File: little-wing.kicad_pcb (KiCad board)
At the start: 2 copper layers, 116.8 x 96 mm, 72 parts, among them IC1 AP7335-WG-7, J1 nice!view, J2 Battery, J3 trackball, J4 trackball, SW1 Power, SW2 Reset, U1 nice!nano v2, U2 PMW3610

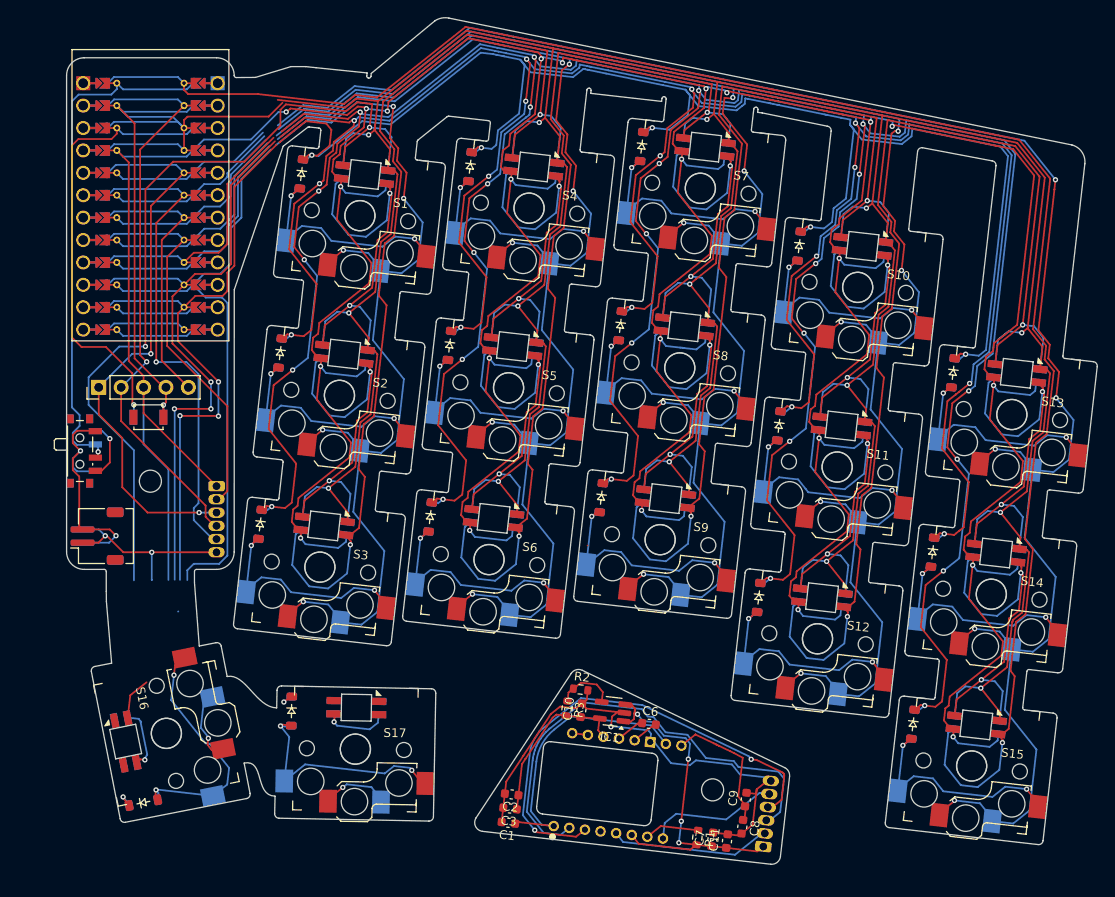
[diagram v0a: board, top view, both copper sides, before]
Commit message: Finalizing the wiring
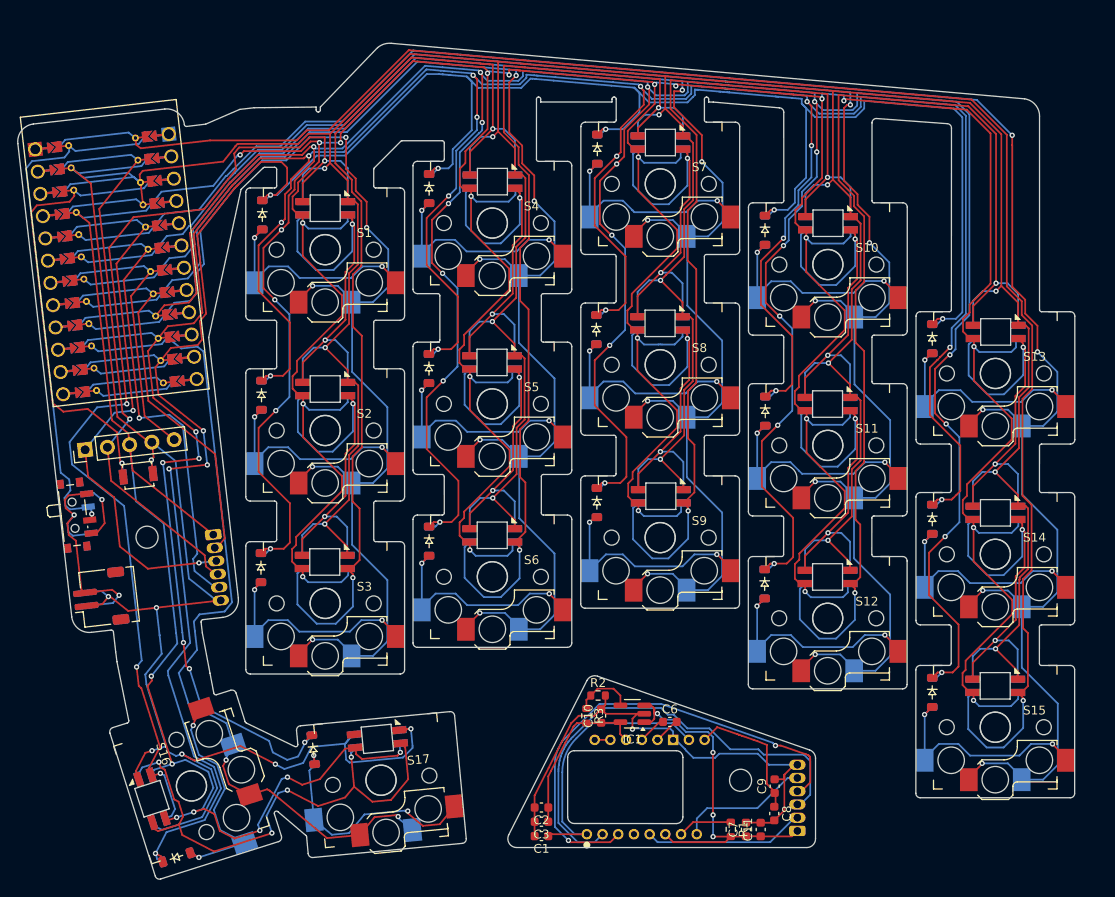
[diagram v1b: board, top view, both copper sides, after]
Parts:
- moved U1 7.63 mm to (102.3, 74.2), turned to -83.5 degrees
- moved SW1 7.28 mm to (97.8, 102.6), turned to -83.5 degrees
- moved D16 7.25 mm to (109.1, 141.4), turned to 18 degrees
- moved J1 7.25 mm to (98.8, 95.2), turned to 96.5 degrees
- moved D19 7.13 mm to (106.4, 134.8), turned to 108 degrees
- moved J2 7.00 mm to (100.5, 112.0), turned to 96.5 degrees
- moved SW2 6.68 mm to (104.8, 98.1), turned to -173.5 degrees
- moved S16 6.61 mm to (110.8, 133.3), turned to 108 degrees
- moved D1 6.42 mm to (118.9, 68.6), turned to -90 degrees
- moved D20 5.88 mm to (126.0, 67.8), turned to -1.80411e-15 degrees
- moved S1 5.51 mm to (126.0, 72.5), turned to -1.80411e-15 degrees
- moved J4 5.51 mm to (113.3, 104.8), turned to -83.5 degrees
- moved D4 5.27 mm to (137.8, 65.6), turned to -90 degrees
- moved D32 5.27 mm to (202.0, 81.9), turned to -1.80411e-15 degrees
- moved D2 5.23 mm to (118.8, 89.0), turned to -90 degrees
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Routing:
- net GND: track 667.7 -> 763.2 mm, vias 19 -> 23
- net Net-(D18-DIN): track 0.00 -> 59.1 mm, vias 0 -> 4
- net VCC: track 629.7 -> 681.9 mm, vias 26 -> 31
- net Row 2: track 248.9 -> 281.6 mm
- net Row 1: track 367.0 -> 391.8 mm, vias 20 -> 22
- net Net-(D19-DIN): track 102.1 -> 121.5 mm, vias 2 -> 4
- net Col 5: track 86.7 -> 96.6 mm
- net Col 0: track 228.4 -> 230.3 mm
- net Col 1: track 201.3 -> 203.0 mm
- net RESET: track 51.9 -> 53.6 mm
- net Net-(D17-A): track 27.0 -> 28.5 mm
- net Net-(D16-A): track 28.5 -> 27.3 mm
- net Row 0: track 437.4 -> 438.6 mm
- net Col 2: track 177.4 -> 178.5 mm
- net Col 3: track 165.4 -> 166.4 mm
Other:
- board size 116.8 x 96 mm -> 119.8 x 94.8 mm
